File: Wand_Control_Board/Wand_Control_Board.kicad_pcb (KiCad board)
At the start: 2 copper layers, 11 x 38.3 mm, 6 parts, among them J1 Conn_01x03_Socket, J2 Conn_01x03_Socket, J3 Conn_01x03_Socket, J5 Conn_01x05_Socket, J8 Conn_01x02_Socket, U1 ATtiny85-20P

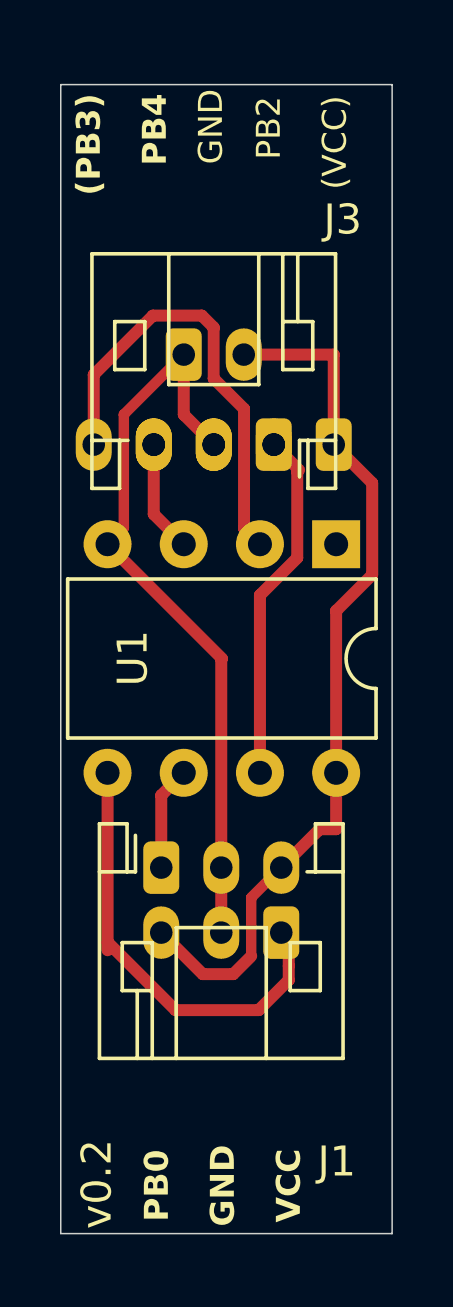
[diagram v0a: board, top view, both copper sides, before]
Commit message: outputs and cleaner silkscreen
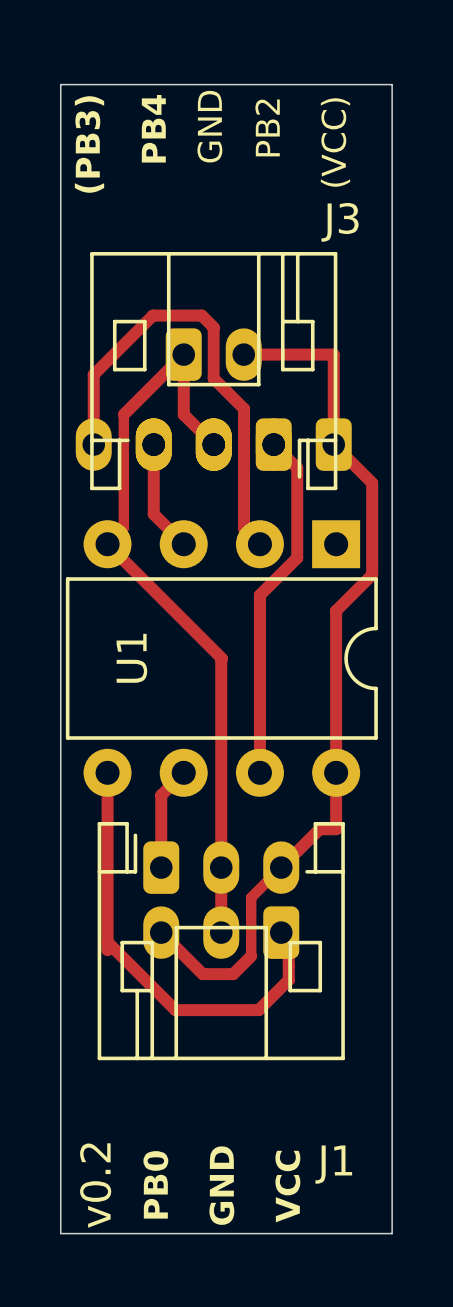
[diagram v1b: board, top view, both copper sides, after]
